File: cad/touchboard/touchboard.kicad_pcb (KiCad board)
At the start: 2 copper layers, 170.1 x 90.1 mm, 55 parts, among them J1 Conn_01x02, J2 Conn_01x02, J3 Conn_01x02, J4 Conn_01x04, J8 Conn_01x02, Q1 PN2222A, Q2 PN2222A, Q3 IRLZ44N, U2 LM2596, U3 ESP32-DEVKIT-V1, U4 adafruit-MAX98357, U5 adafruit-MAX98357

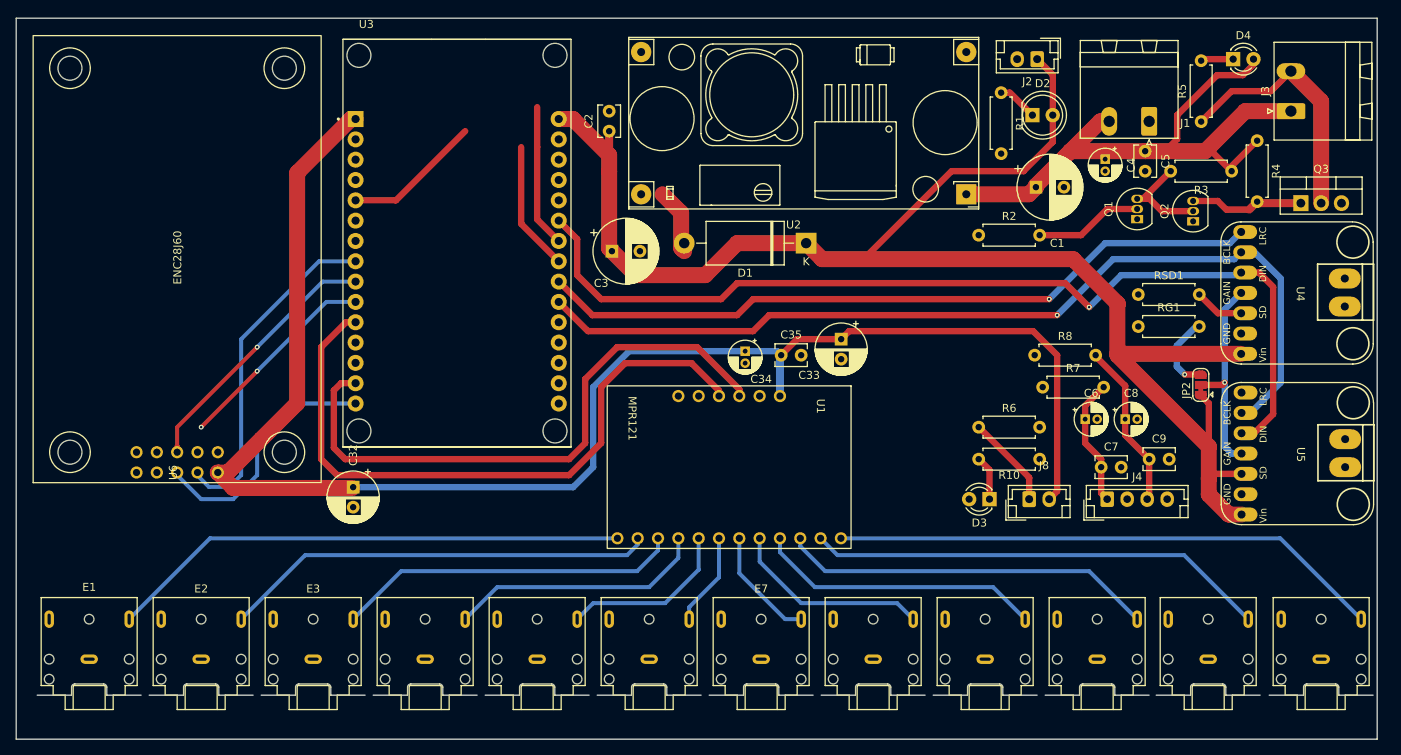
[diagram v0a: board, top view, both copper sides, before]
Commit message: pcb done
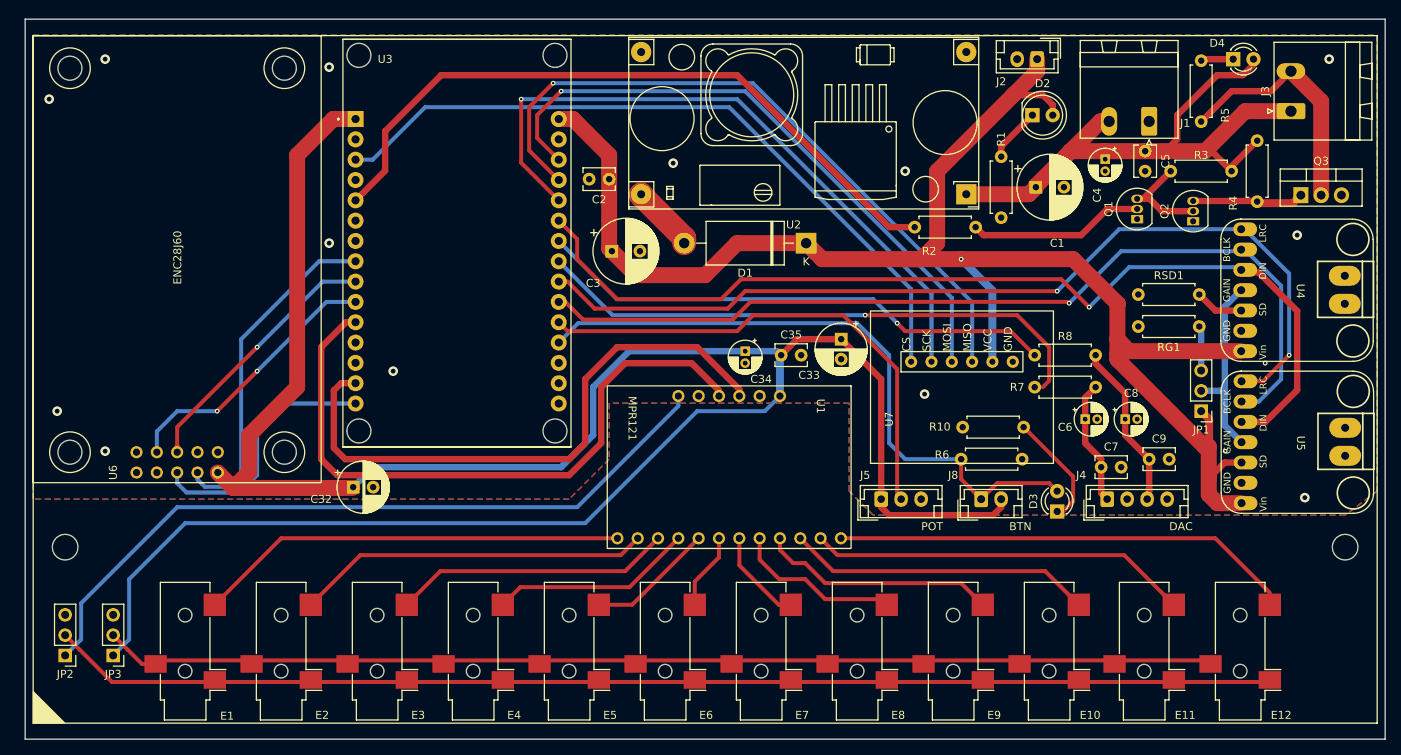
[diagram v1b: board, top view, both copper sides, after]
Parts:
- added H1: MountingHole, MountingHole:MountingHole_3.2mm_M3, F.Cu at (46.0, 107.0)
- added H2: MountingHole, MountingHole:MountingHole_3.2mm_M3, F.Cu at (206.0, 107.0)
- added J5: Conn_01x03, Connector_JST:JST_EH_B3B-EH-A_1x03_P2.50mm_Vertical, F.Cu at (148.0, 101.0)
- added JP1: Jumper_3_Open, Connector_PinHeader_2.54mm:PinHeader_1x03_P2.54mm_Vertical, F.Cu at (188.0, 90.0)
- added JP3: Jumper_3_Open, Connector_PinHeader_2.54mm:PinHeader_1x03_P2.54mm_Vertical, F.Cu at (52.0, 120.5)
- added U7: ~, SD:SD_module, F.Cu at (146.7, 83.8)
- E1, E10, E11, E12, E2, E3, E4, E5, E6, E7, E8, E9: footprint Connector_Audio:Jack_3.5mm_CUI_SJ1-3523N_Horizontal -> Connector_Audio:Jack_3.5mm_CUI_SJ-3523-SMT_Horizontal
- JP2: value SolderJumper_3_Bridged12 -> Jumper_3_Open; footprint Jumper:SolderJumper-3_P1.3mm_Bridged12_RoundedPad1.0x1.5mm -> Connector_PinHeader_2.54mm:PinHeader_1x03_P2.54mm_Vertical
- moved JP2 145.9 mm to (46.0, 120.5), turned to 180 degrees
- moved E1 12.0 mm to (61.0, 120.0), turned to 180 degrees
- moved E12 10.2 mm to (192.9, 120.0), turned to 180 degrees
- moved E2 10.0 mm to (73.0, 120.0), turned to 180 degrees
- moved D3 8.60 mm to (170.0, 102.5), turned to 90 degrees
- moved E11 8.06 mm to (180.9, 120.0), turned to 180 degrees
- moved E3 8.06 mm to (85.0, 120.0), turned to 180 degrees
- moved R2 8.06 mm to (152.2, 67.0)
- moved R1 8.00 mm to (163.0, 58.2)
- moved R10 6.90 mm to (165.8, 92.0), turned to 180 degrees
- moved E10 6.08 mm to (169.0, 120.0), turned to 180 degrees
- moved E4 6.08 mm to (97.0, 120.0), turned to 180 degrees
- moved C2 6.00 mm to (114.0, 61.0), turned to 180 degrees
- moved J8 6.00 mm to (160.5, 101.0)
- moved R6 4.56 mm to (158.0, 96.0)
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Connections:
- E1 pad R: +3.3V -> SVCC
- E1 pad S: GND -> SGND
- E10 pad R: +3.3V -> SVCC
- E10 pad S: GND -> SGND
- E11 pad R: +3.3V -> SVCC
- E11 pad S: GND -> SGND
- E12 pad R: +3.3V -> SVCC
- E12 pad S: GND -> SGND
- E2 pad R: +3.3V -> SVCC
- E2 pad S: GND -> SGND
- E3 pad R: +3.3V -> SVCC
- E3 pad S: GND -> SGND
- E4 pad R: +3.3V -> SVCC
- E4 pad S: GND -> SGND
- E5 pad R: +3.3V -> SVCC
- E5 pad S: GND -> SGND
- E6 pad R: +3.3V -> SVCC
- E6 pad S: GND -> SGND
- E7 pad R: +3.3V -> SVCC
- E7 pad S: GND -> SGND
- E8 pad R: +3.3V -> SVCC
- E8 pad S: GND -> SGND
- E9 pad R: +3.3V -> SVCC
- E9 pad S: GND -> SGND
- JP2 pad 1: +5V -> GND
- JP2 pad 2: GAIN -> SGND
- JP2 pad 3: Net-(JP2-B) -> unconnected-(JP2-B-Pad3)
- RG1 pad 2: Net-(JP2-B) -> Net-(JP1-B)
- U3 pad 19: unconnected-(U3-D34-Pad19) -> BTN1
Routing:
- net SGND: track 0.00 -> 155.4 mm
- net SVCC: track 0.00 -> 142.8 mm
- net GND: track 0.00 -> 93.5 mm, vias 0 -> 15
- net +3.3V: track 197.2 -> 290.6 mm
- net HSPI_CS: track 0.00 -> 90.7 mm
- net HSPI_MISO: track 0.00 -> 86.0 mm, vias 0 -> 1
- net HSPI_CLK: track 0.00 -> 84.5 mm, vias 0 -> 1
- net HSPI_MOSI: track 0.00 -> 78.5 mm, vias 0 -> 1
- net BTN1: track 11.6 -> 81.6 mm
- net LED_PWM1: track 17.3 -> 87.1 mm
- net POT_GAIN: track 0.00 -> 62.8 mm
- net DAC1: track 16.2 -> 71.1 mm, vias 0 -> 1
- net DAC2: track 17.8 -> 65.4 mm, vias 0 -> 1
- net LRC: track 91.3 -> 116.8 mm, vias 1 -> 2
- net +5V: track 193.7 -> 209.7 mm, vias 0 -> 1
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- added copper zone on B.Cu, net GND
- added copper zone on F.Cu, net GND
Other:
- board size 170.1 x 90.1 mm -> 170 x 90 mm
- board text added: "BTN"
- board text added: "DAC"
- board text added: "POT"
